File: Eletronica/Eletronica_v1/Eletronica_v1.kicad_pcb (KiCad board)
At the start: 2 copper layers, 50 x 90 mm, 33 parts, among them J1 Motor_R, J2 Motor_L, J3 Sharp_G2Y0A41SK, J4 Sharp_G2Y0A41SK, J5 Sharp_G2Y0A41SK, J6 Bateria, SW1 TROCA_MODO, SW2 SW_SPDT, U1 QTR-1A_REFLECTANCE_SENSOR, U3 TSOP1838, U4 QTR-1A_REFLECTANCE_SENSOR, U5 Mini560, U6 ROB-14450

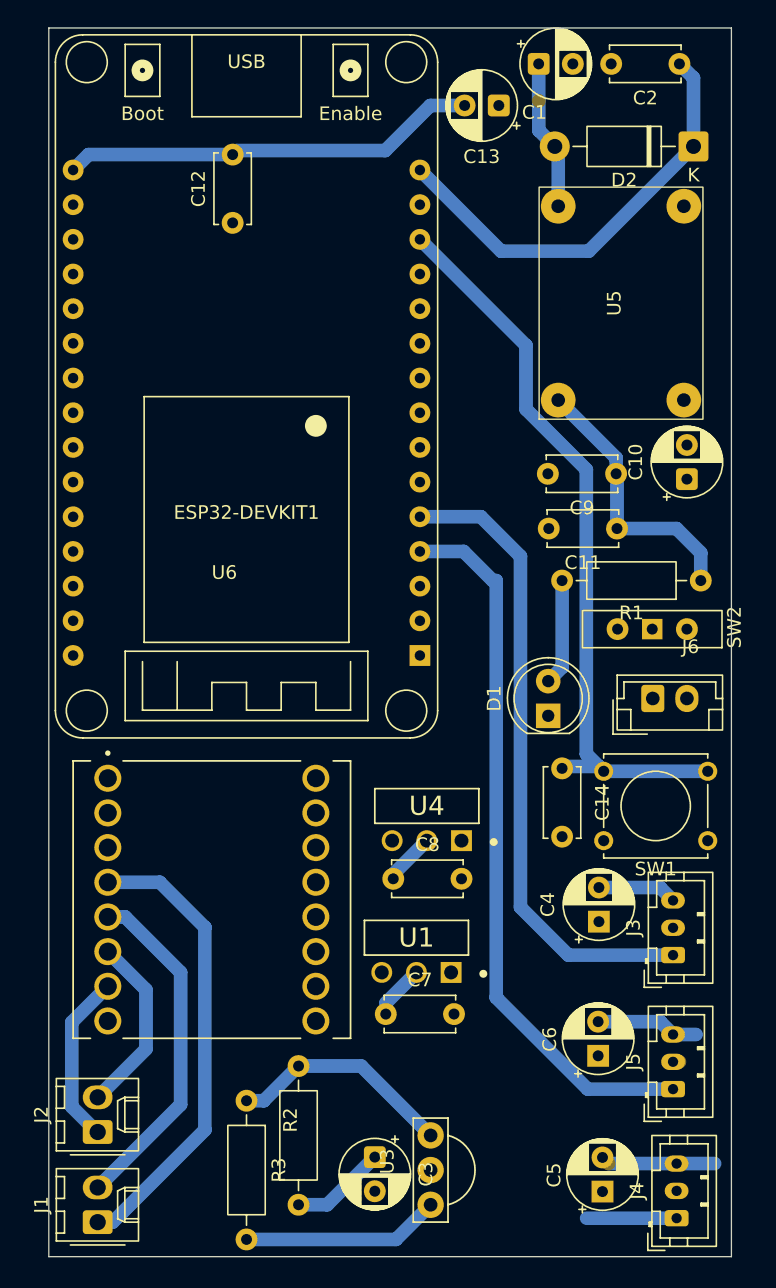
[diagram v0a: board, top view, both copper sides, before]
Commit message: Finalizado a versao funcional da placa
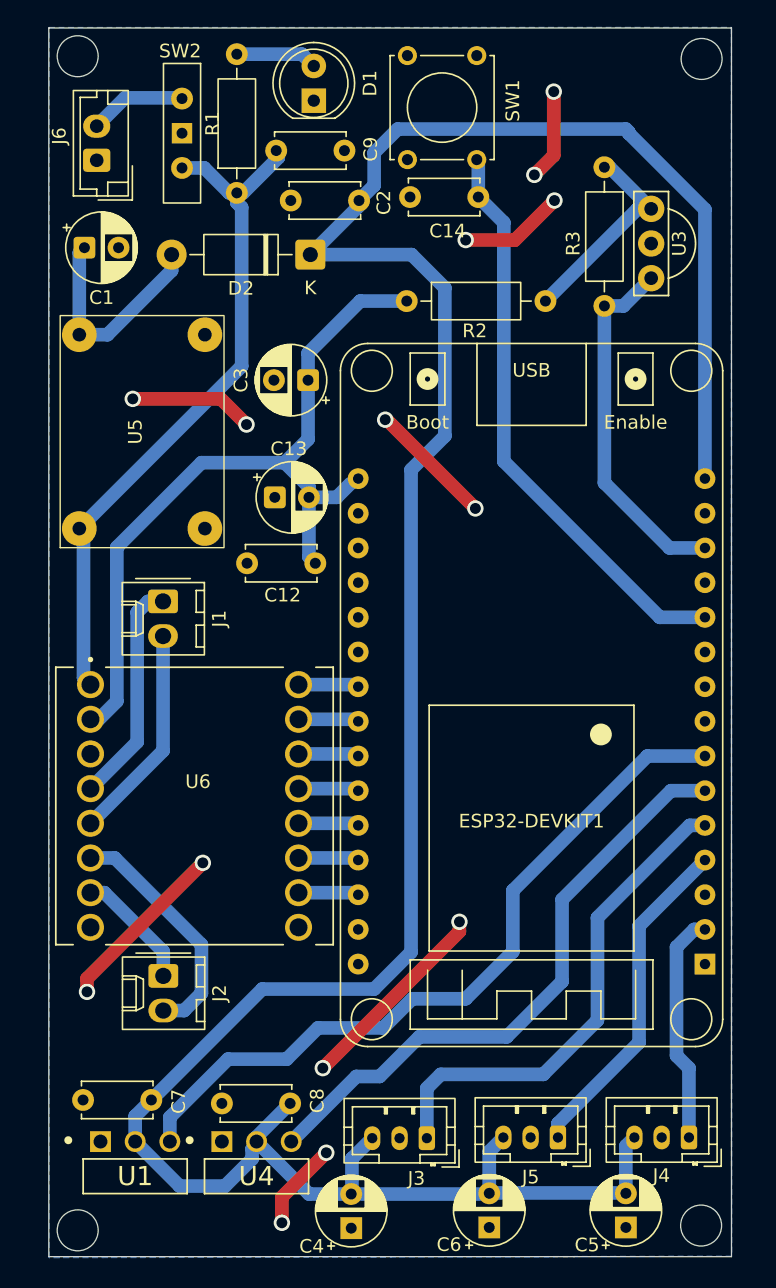
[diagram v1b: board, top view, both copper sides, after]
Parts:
- removed C10: 10uF, Capacitor_THT:CP_Radial_D5.0mm_P2.50mm
- removed C11: 100nF, Capacitor_THT:C_Disc_D5.0mm_W2.5mm_P5.00mm
- moved R3 73.2 mm to (84.4, 46.4)
- moved U3 69.8 mm to (87.8, 52.0)
- moved R2 66.7 mm to (69.9, 56.2), turned to 0 degrees
- moved C3 57.1 mm to (62.7, 62.0), turned to 180 degrees
- moved J6 56.7 mm to (47.2, 45.9), turned to 90 degrees
- moved SW1 54.5 mm to (70.0, 45.9), turned to 90 degrees
- moved SW2 50.1 mm to (53.4, 43.9), turned to -90 degrees
- moved D1 48.2 mm to (63.1, 41.6)
- moved J1 45.7 mm to (52.0, 78.2), turned to -90 degrees
- moved R1 44.3 mm to (57.5, 48.3), turned to 90 degrees
- moved C14 42.3 mm to (75.1, 48.6), turned to 180 degrees
- moved U5 36.3 mm to (50.5, 65.8)
- moved C1 35.9 mm to (46.3, 52.3)
- moved C9 34.4 mm to (60.3, 45.2), turned to 0 degrees
- moved C13 33.1 mm to (60.2, 70.6), turned to 0 degrees
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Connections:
- ESP32-DEVKIT1 pad 11: unconnected-(ESP32-DEVKIT1-ADC2_6/14-Pad11) -> MODE_SWT
- ESP32-DEVKIT1 pad 13: MODE_SWT -> INFRA_OUT
- ESP32-DEVKIT1 pad 22: unconnected-(ESP32-DEVKIT1-TXD_2/17-Pad22) -> PWM_MOTOR_R
- ESP32-DEVKIT1 pad 23: unconnected-(ESP32-DEVKIT1-SS/5-Pad23) -> MOTOR_R_IN2
- ESP32-DEVKIT1 pad 24: PWM_MOTOR_R -> MOTOR_R_IN1
- ESP32-DEVKIT1 pad 25: MOTOR_R_IN1 -> STBY
- ESP32-DEVKIT1 pad 26: MOTOR_R_IN2 -> MOTOR_L_IN1
- ESP32-DEVKIT1 pad 27: unconnected-(ESP32-DEVKIT1-RXD_0/3-Pad27) -> MOTOR_L_IN2
- ESP32-DEVKIT1 pad 28: unconnected-(ESP32-DEVKIT1-TXD_0/1-Pad28) -> PWM_MOTOR_L
- ESP32-DEVKIT1 pad 29: PWM_MOTOR_L -> unconnected-(ESP32-DEVKIT1-SCL/22-Pad29)
- ESP32-DEVKIT1 pad 30: MOTOR_L_IN1 -> unconnected-(ESP32-DEVKIT1-MOSI/23-Pad30)
- ESP32-DEVKIT1 pad 8: MOTOR_L_IN2 -> unconnected-(ESP32-DEVKIT1-ADC2_8/25-Pad8)
- ESP32-DEVKIT1 pad 9: STBY -> unconnected-(ESP32-DEVKIT1-ADC2_9/26-Pad9)
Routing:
- net VCC 5V: track 61.1 -> 202.5 mm
- net GND: track 1.28 -> 67.4 mm, vias 0 -> 14
- net QTR_R: track 0.00 -> 54.6 mm
- net QTR_L: track 0.00 -> 44.5 mm
- net BAT: track 20.1 -> 50.7 mm
- net IR_F: track 52.7 -> 24.8 mm
- net 3V3: track 37.3 -> 57.9 mm
- net Net-(J1-Pin_1): track 34.0 -> 16.6 mm
- net MODE_SWT: track 55.5 -> 42.4 mm
- net INFRA_OUT: track 14.5 -> 26.6 mm
- net IR_R: track 46.9 -> 36.4 mm
- net IR_L: track 6.59 -> 16.9 mm
- net Net-(J1-Pin_2): track 25.3 -> 15.9 mm
- net Net-(J6-Pin_2): track 0.00 -> 7.13 mm
- net Net-(D2-A): track 11.0 -> 16.4 mm
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- added copper zone on B.Cu, net GND
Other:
- outline, holes or cut-outs redrawn
